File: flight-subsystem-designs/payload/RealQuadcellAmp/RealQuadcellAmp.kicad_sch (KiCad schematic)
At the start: 91 parts, among them J1 Screw_Terminal_01x02, J2 Conn_01x04_Pin, J3 Conn_01x04_Pin, U1 LM2904, U2 LM2904, U3 LM2904, U4 LM2904, U6 LM2904, U7 L78L33_SOT89

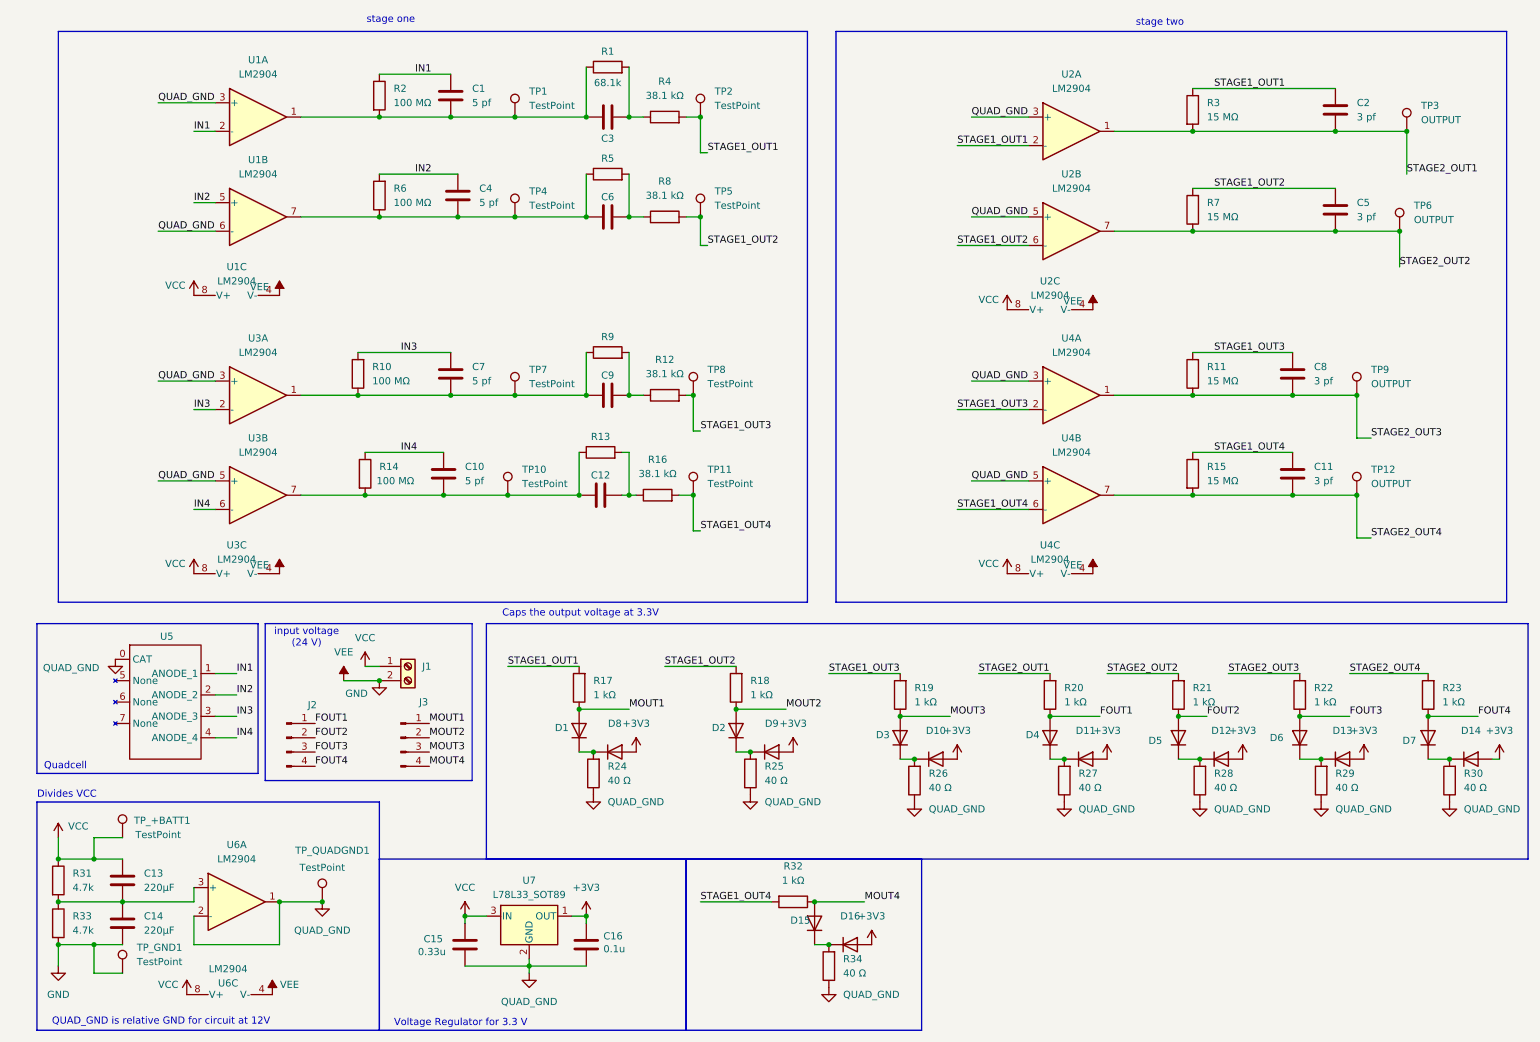
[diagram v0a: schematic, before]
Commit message: new quadcell rev
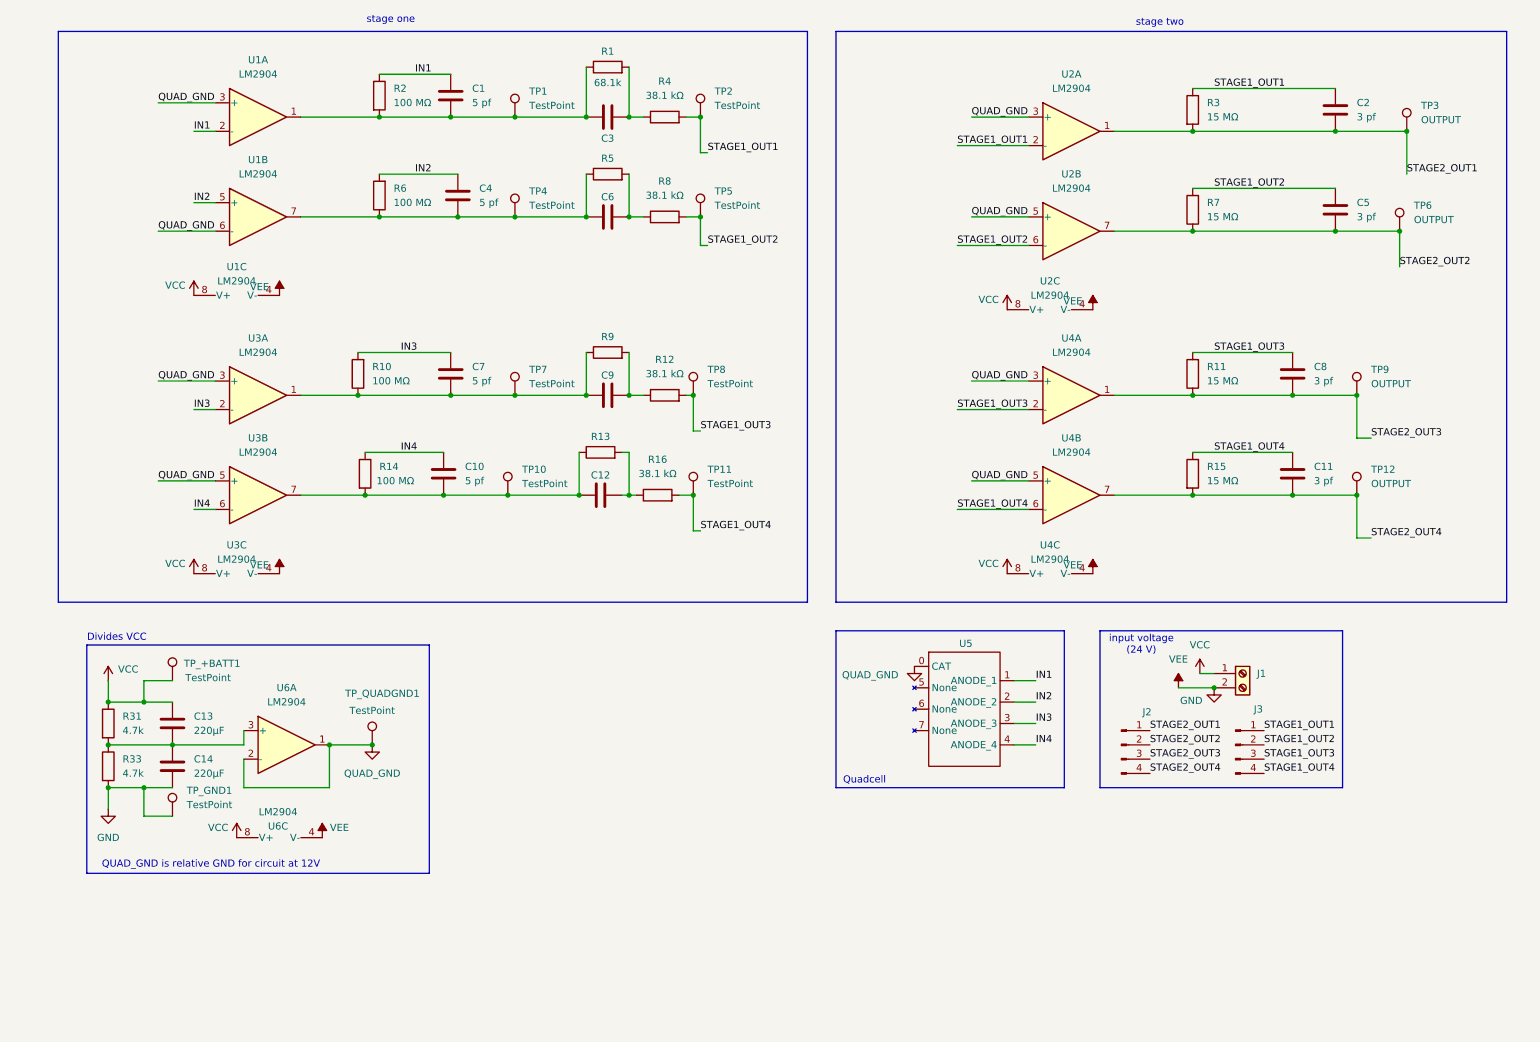
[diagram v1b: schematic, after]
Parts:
- removed C15: 0.33u, Capacitor_SMD:C_0805_2012Metric_Pad1.18x1.45mm_HandSolder, symbol Device:C
- removed C16: 0.1u, Capacitor_SMD:C_0805_2012Metric_Pad1.18x1.45mm_HandSolder, symbol Device:C
- removed D1, D10, D11, D12, D13, D14, D15, D16, D2, D3, D4, D5, D6, D7, D8, D9: ~, Diode_SMD:D_0805_2012Metric_Pad1.15x1.40mm_HandSolder, symbol Diode:1N4001
- removed R17, R18, R19, R20, R21, R22, R23, R32: 1 kΩ, Resistor_SMD:R_0805_2012Metric_Pad1.20x1.40mm_HandSolder, symbol Device:R
- removed R24, R25, R26, R27, R28, R29, R30, R34: 40 Ω, Resistor_SMD:R_0805_2012Metric_Pad1.20x1.40mm_HandSolder, symbol Device:R
- removed U7: L78L33_SOT89, Package_TO_SOT_SMD:SOT-89-3, symbol Regulator_Linear:L78L33_SOT89
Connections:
- net FOUT1 is gone; now on net STAGE2_OUT1: J2.1 (Pin_1)
- net FOUT2 is gone; now on net STAGE2_OUT2: J2.2 (Pin_2)
- net FOUT3 is gone; now on net STAGE2_OUT3: J2.3 (Pin_3)
- net FOUT4 is gone; now on net STAGE2_OUT4: J2.4 (Pin_4)
- net MOUT1 is gone; now on net STAGE1_OUT1: J3.1 (Pin_1)
- net MOUT2 is gone; now on net STAGE1_OUT2: J3.2 (Pin_2)
- net MOUT3 is gone; now on net STAGE1_OUT3: J3.3 (Pin_3)
- net MOUT4 is gone; now on net STAGE1_OUT4: J3.4 (Pin_4)
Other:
- note removed: "Caps the output voltage at 3.3V"
- note removed: "Voltage Regulator for 3.3 V"
- moved on the sheet: C13, C14, J1, J2, J3, R31, R33, TP_+BATT1, TP_GND1, TP_QUADGND1, U5, U6A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
